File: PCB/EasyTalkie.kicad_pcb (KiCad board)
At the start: 2 copper layers, 55.2 x 81.8 mm, 6 parts, among them SW1 SW_Push, SW2 ON/OFF, U1 XIAO-ESP32-S3-DIP, U2 INMP441, U3 MAX98357A

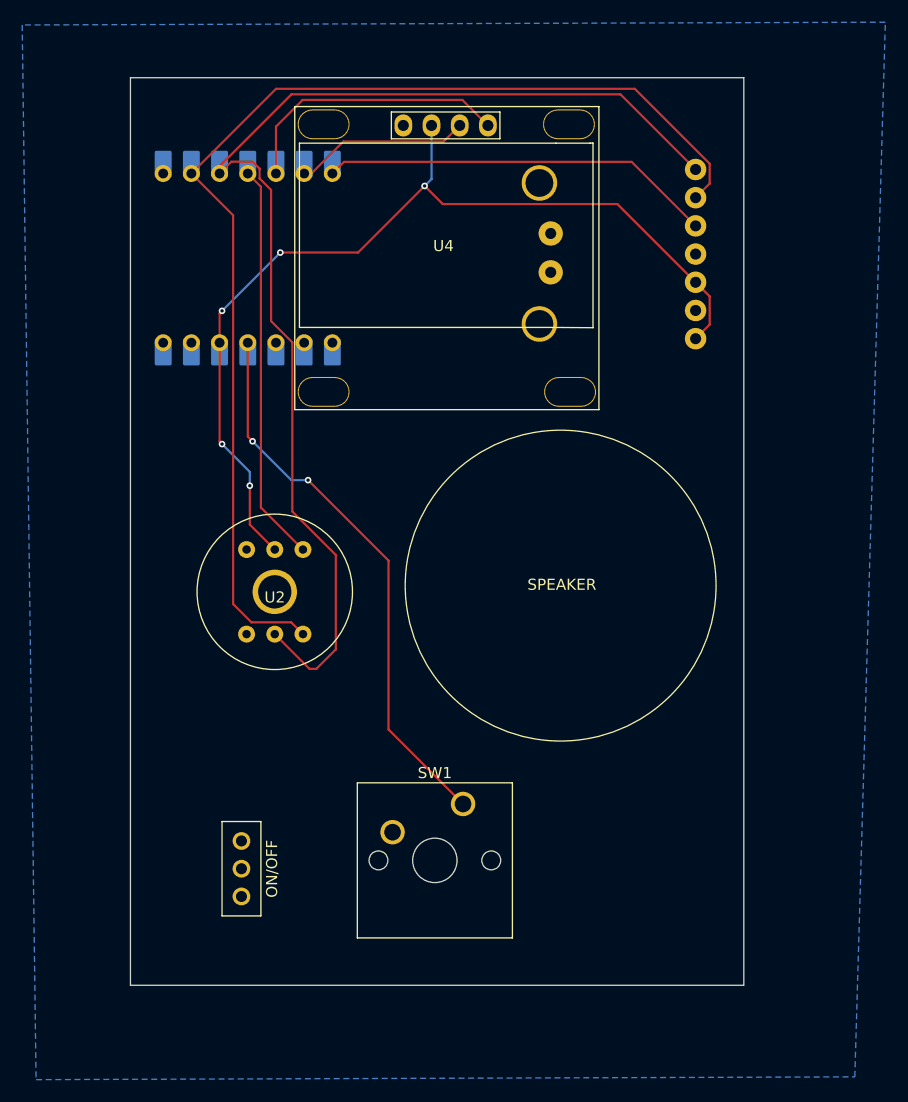
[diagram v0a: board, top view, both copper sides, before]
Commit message: cad
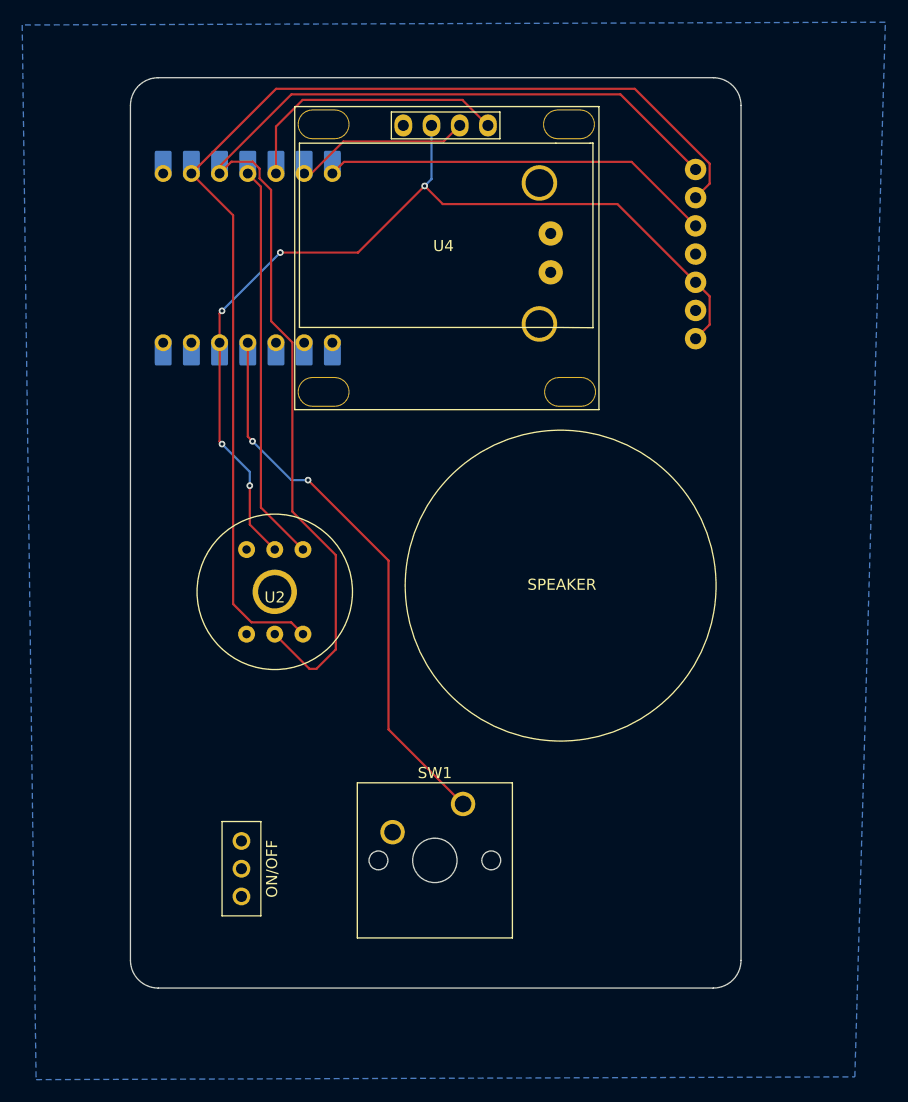
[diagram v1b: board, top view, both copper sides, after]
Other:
- board size 55.2 x 81.8 mm -> 55 x 82 mm
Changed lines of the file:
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@@
 		(layer "F.SilkS")
 	)
-	(gr_rect
-		(start 188 23.5)
-		(end 243.25 105.25)
+	(gr_arc
+		(start 190.5 105.5)
+		(mid 188.732233 104.767767)
+		(end 188 103)
 		(stroke
 			(width 0.05)
 			(type default)
 		)
-		(fill no)
 		(layer "Edge.Cuts")
 	)
+	(gr_line
+		(start 240.5 105.5)
+		(end 190.5 105.5)
+		(stroke
+			(width 0.05)
+			(type default)
+		)
+		(layer "Edge.Cuts")
+	)
+	(gr_line
+		(start 190.5 23.5)
+		(end 240.5 23.5)
+		(stroke
+			(width 0.05)
+			(type default)
+		)
+		(layer "Edge.Cuts")
+	)
+	(gr_line
+		(start 188 103)
+		(end 188 26)
+		(stroke
+			(width 0.05)
+			(type default)
+		)
+		(layer "Edge.Cuts")
+	)
+	(gr_arc
+		(start 243 103)
+		(mid 242.267767 104.767767)
+		(end 240.5 105.5)
+		(stroke
+			(width 0.05)
+			(type default)
+		)
+		(layer "Edge.Cuts")
+	)
+	(gr_arc
+		(start 240.5 23.5)
+		(mid 242.267767 24.232233)
+		(end 243 26)
+		(stroke
+			(width 0.05)
+			(type default)
+		)
+		(layer "Edge.Cuts")
+	)
+	(gr_arc
+		(start 188 26)
+		(mid 188.732233 24.232233)
+		(end 190.5 23.5)
+		(stroke
+			(width 0.05)
+			(type default)
+		)
+		(layer "Edge.Cuts")
+	)
+	(gr_line
+		(start 243 26)
+		(end 243 103)
+		(stroke
+			(width 0.05)
+			(type default)
+		)
+		(layer "Edge.Cuts")
+	)
